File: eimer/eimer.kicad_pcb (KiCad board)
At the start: 2 copper layers, 21 x 51 mm, 33 parts, among them J1 Conn_01x20, J2 Conn_01x20, J3 Conn_01x03, J4 USB_C_Receptacle_USB2.0_14P, SW1 SW_Push, U1 RP2040, U2 MCP1700x-330xxTT, U4 W25Q16JVUXIQ TR, Y1 12 MHz

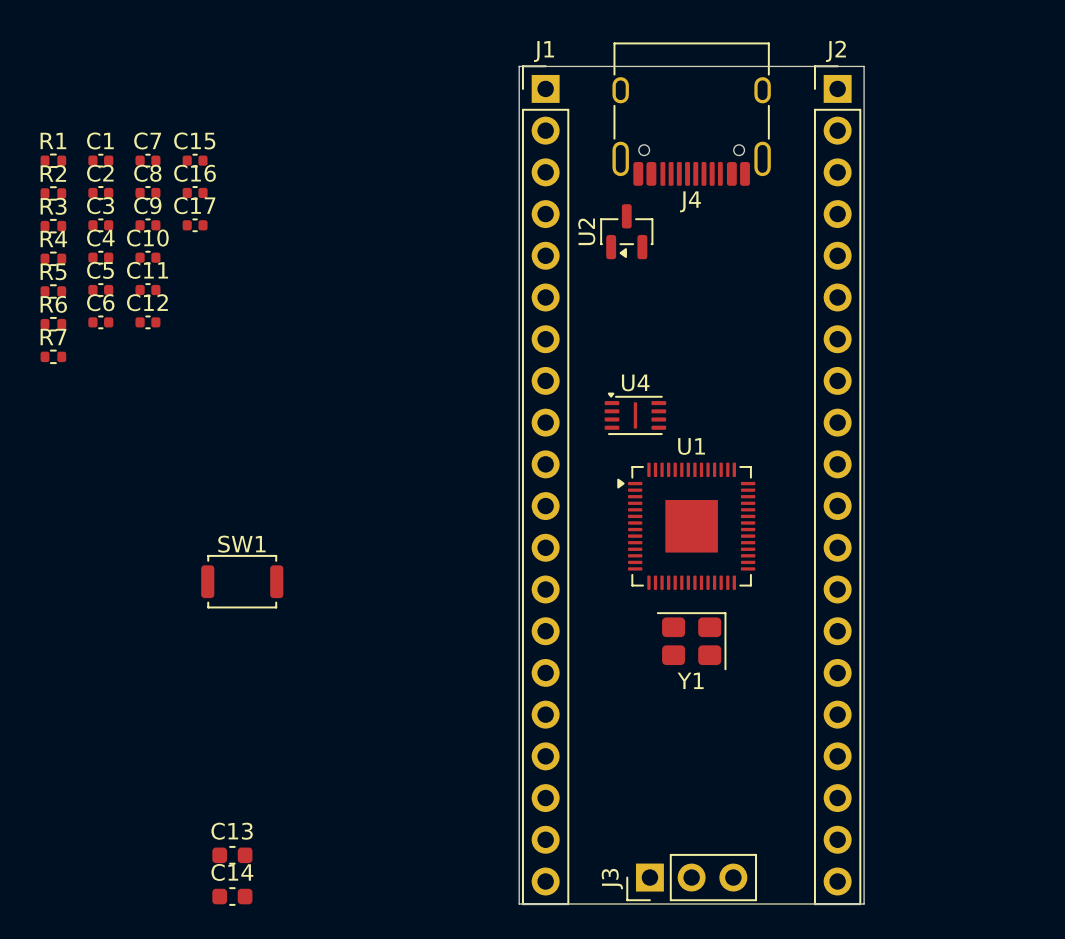
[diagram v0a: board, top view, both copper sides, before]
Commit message: placed more caps
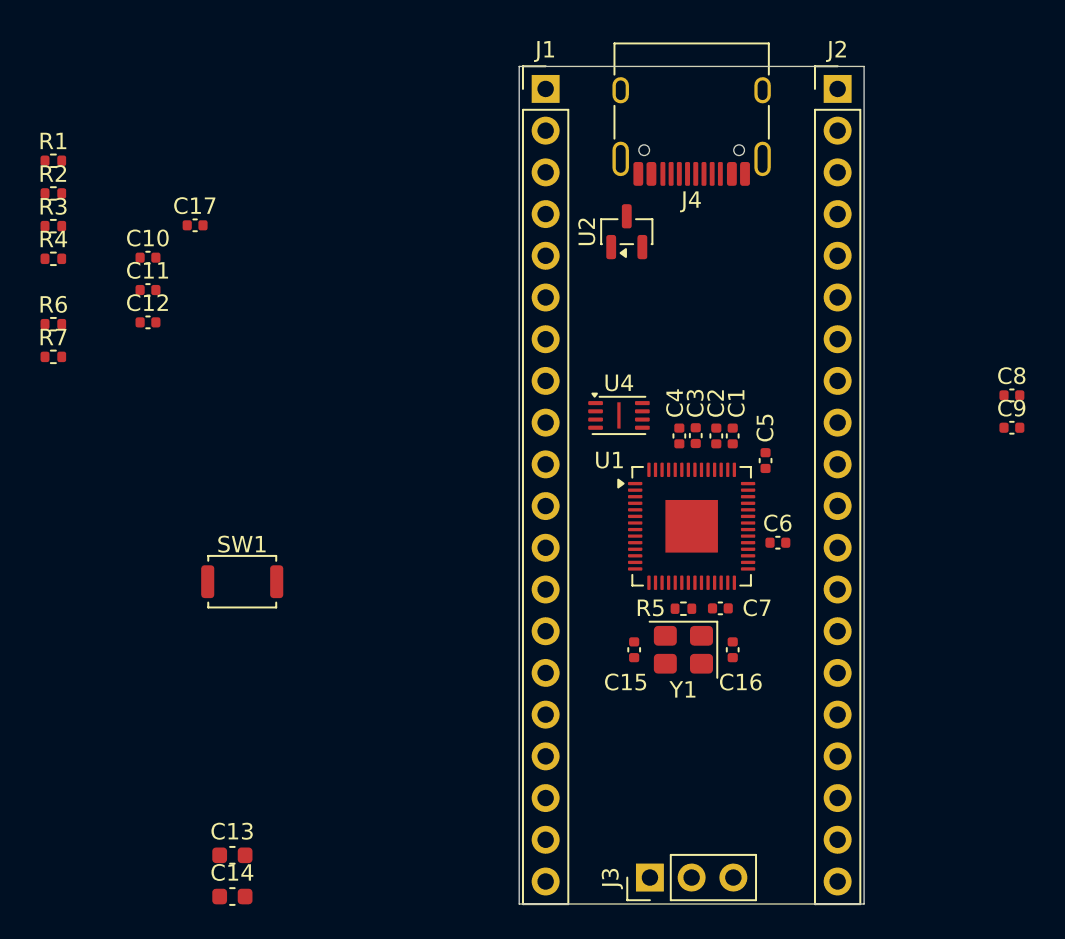
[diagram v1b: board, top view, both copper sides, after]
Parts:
- moved C8 54.0 mm to (182.0, 84.0)
- moved C9 54.0 mm to (182.0, 86.0)
- moved C7 44.3 mm to (164.2, 97.0)
- moved C6 43.4 mm to (167.8, 93.0)
- moved C16 43.0 mm to (165.0, 99.5), turned to -90 degrees
- moved R5 43.0 mm to (162.0, 97.0)
- moved C1 42.0 mm to (165.0, 86.5), turned to 90 degrees
- moved C5 41.8 mm to (167.0, 88.0), turned to 90 degrees
- moved C2 40.3 mm to (164.0, 86.5), turned to 90 degrees
- moved C15 40.0 mm to (159.0, 99.5), turned to -90 degrees
- moved C3 38.4 mm to (162.8, 86.5), turned to 90 degrees
- moved C4 36.9 mm to (161.8, 86.5), turned to 90 degrees
- moved U4 1.00 mm to (158.1, 85.2)
- moved Y1 0.72 mm to (162.0, 99.5)

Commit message: go to shleeep
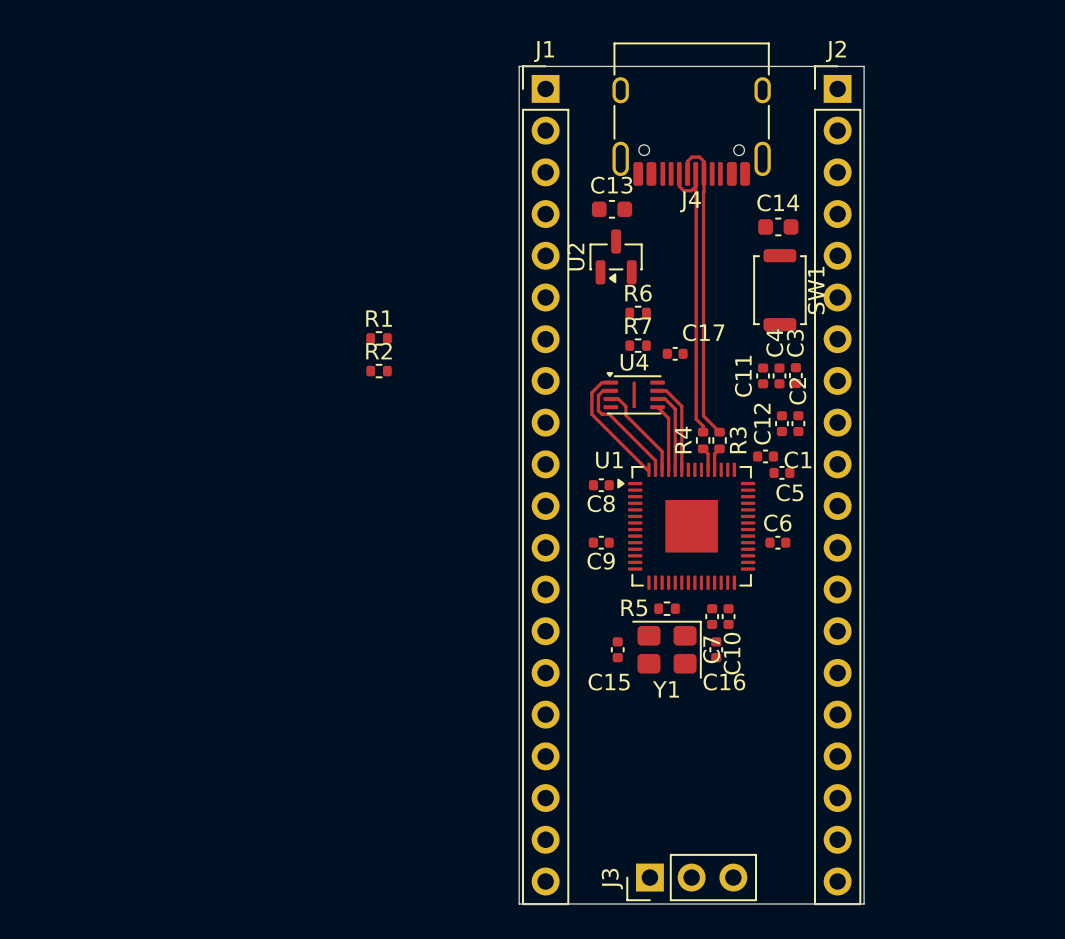
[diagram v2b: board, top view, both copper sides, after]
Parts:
- moved C14 52.6 mm to (167.8, 73.8)
- moved C13 45.6 mm to (157.7, 72.7)
- moved R3 42.6 mm to (164.2, 86.8), turned to -90 degrees
- moved C10 41.6 mm to (164.8, 97.5), turned to -90 degrees
- moved R4 41.1 mm to (163.2, 86.8), turned to 90 degrees
- moved C12 39.1 mm to (168.0, 85.8), turned to 90 degrees
- moved C11 37.8 mm to (166.8, 82.8), turned to 90 degrees
- moved SW1 37.2 mm to (167.9, 77.6), turned to -90 degrees
- moved R7 35.6 mm to (159.2, 81.0)
- moved R6 35.6 mm to (159.2, 79.0)
- moved C17 30.3 mm to (161.5, 81.5)
- moved C9 26.0 mm to (157.0, 93.0), turned to 180 degrees
- moved C8 25.6 mm to (157.0, 89.5), turned to 180 degrees
- moved R1 22.6 mm to (143.5, 80.6)
- moved R2 22.6 mm to (143.5, 82.5)
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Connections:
- U1 pad 23: +3.3V -> +1V1
- U1 pad 43: +1V1 -> +3.3V
- U1 pad 45: +3.3V -> +1V1
- U1 pad 48: +1V1 -> +3.3V
- U1 pad 50: +3.3V -> +1V1
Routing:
- net USB_D-: track 0.00 -> 18.9 mm
- net USB_D+: track 0.00 -> 18.6 mm
- net QSPI_SS: track 0.00 -> 7.60 mm
- net QSPI_SD1: track 0.00 -> 7.09 mm
- net QSPI_SD2: track 0.00 -> 5.88 mm
- net QSPI_SD3: track 0.00 -> 5.73 mm
- net QSPI_SCLK: track 0.00 -> 5.03 mm
- net QSPI_SD0: track 0.00 -> 4.09 mm
- net Net-(U1-USB_DP): track 0.00 -> 1.40 mm
- net Net-(U1-USB_DM): track 0.00 -> 1.40 mm
